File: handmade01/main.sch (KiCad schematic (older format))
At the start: 69 parts, among them CON1 MicroSD, CON2 MicroSD, J1 JACK_TRS_6PINS, P1 VOLUMN, P4 USB_OTG, P6 UART_DEBUG, Q1 1AM, SW1 POWER, SW10 R, SW11 A, SW12 B, SW13 X, SW14 Y, SW2 Reset, SW3 UP, SW4 Down, SW5 Left, SW6 Right, SW7 Select, SW8 Start, SW9 L, U1 PCM5102A, U2 PAM8403, U3 IPS_2.4_240x320_ST7789V, U4 CM3354, U5 TPS71718

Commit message: 20171130
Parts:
- J1: footprint Connectors:PJ311_3.5mm_Jack -> mylib:pj311_3.5mm
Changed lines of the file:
@@
 F 0 "J1" H 1800 10200 50  0000 C CNN
 F 1 "JACK_TRS_6PINS" H 1750 9500 50  0000 C CNN
-F 2 "Connectors:PJ311_3.5mm_Jack" H 1900 9650 50  0000 C CNN
+F 2 "mylib:pj311_3.5mm" H 1900 9650 50  0000 C CNN
 F 3 "" H 1900 9650 50  0000 C CNN
 	1    1800 9800

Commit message: 20171201
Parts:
- BAT1, P6: footprint Connectors_Molex:Molex_SPOX-5267_22-03-5035_03x2.54mm_Straight -> Connectors:GS3
- LS1, LS2: footprint Resistors_SMD:R_2010_HandSoldering -> Connectors:GS2
- U3: footprint mylib:fpc-45pin-0.5mm -> mylib:fpc-45pin-0.5mm-down
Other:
- note added: "20171201"
- note removed: "20171130"
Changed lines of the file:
@@
 handmade01
 Text Notes 13000 11050 0    60   ~ 12
-20171130
+20171201
 $Comp
 L +5V #PWR05
@@
 F 0 "U3" H 4150 1850 60  0000 C CNN
 F 1 "IPS_2.4_240x320_ST7789V" H 4700 1750 60  0000 C CNN
-F 2 "mylib:fpc-45pin-0.5mm" H 5150 1500 60  0000 C CNN
+F 2 "mylib:fpc-45pin-0.5mm-down" H 5150 1500 60  0000 C CNN
 F 3 "" H 5150 1500 60  0000 C CNN
 	1    5900 1500
@@
 F 0 "P6" H 11200 1750 50  0000 C CNN
 F 1 "UART_DEBUG" V 11300 1550 50  0000 C CNN
-F 2 "Connectors_Molex:Molex_SPOX-5267_22-03-5035_03x2.54mm_Straight" H 11200 1550 50  0000 C CNN
+F 2 "Connectors:GS3" H 11200 1550 50  0000 C CNN
 F 3 "" H 11200 1550 50  0000 C CNN
 	1    11200 1550
@@
 F 0 "LS2" H 4050 10325 50  0000 R CNN
 F 1 "SPEAKER_L" H 4050 10250 50  0000 R CNN
-F 2 "Resistors_SMD:R_2010_HandSoldering" H 4000 9900 50  0000 C CNN
+F 2 "Connectors:GS2" H 4000 9900 50  0000 C CNN
 F 3 "" H 3990 10050 50  0000 C CNN
 	1    4000 10100
@@
 F 0 "LS1" H 4050 9675 50  0000 R CNN
 F 1 "SPEAKER_R" H 4050 9600 50  0000 R CNN
-F 2 "Resistors_SMD:R_2010_HandSoldering" H 4000 9250 50  0000 C CNN
+F 2 "Connectors:GS2" H 4000 9250 50  0000 C CNN
 F 3 "" H 3990 9400 50  0000 C CNN
 	1    4000 9450
@@
 F 0 "BAT1" H 7600 10150 50  0000 L CNN
 F 1 "BAT" H 7600 10050 50  0000 L CNN
-F 2 "Connectors_Molex:Molex_SPOX-5267_22-03-5035_03x2.54mm_Straight" V 7500 10110 50  0000 C CNN
+F 2 "Connectors:GS3" V 7500 10110 50  0000 C CNN
 F 3 "" V 7500 10110 50  0000 C CNN
 	1    7500 10050

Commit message: 20171204
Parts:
- P4: footprint Connectors:USB_Micro-B -> Connectors:USB_Mini-B
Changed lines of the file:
@@
 F 0 "P4" H 6725 9675 50  0000 C CNN
 F 1 "USB_OTG" H 6400 10000 50  0000 C CNN
-F 2 "Connectors:USB_Micro-B" V 6350 9700 50  0000 C CNN
+F 2 "Connectors:USB_Mini-B" V 6350 9700 50  0000 C CNN
 F 3 "" V 6350 9700 50  0000 C CNN
 	1    6400 9800

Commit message: 20171207
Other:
- note added: "Handmade01"
- note removed: "1.0"
- note removed: "20171201"
- note removed: "handmade01"
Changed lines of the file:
@@
 EESchema Schematic File Version 2
-LIBS:main-rescue
 LIBS:power
 LIBS:device
@@
 LIBS:memory
 LIBS:xilinx
+LIBS:special
 LIBS:microcontrollers
 LIBS:dsp
@@
 LIBS:contrib
 LIBS:valves
-LIBS:switches
-LIBS:mysch
 LIBS:main-cache
-EELAYER 25 0
+EELAYER 27 0
 EELAYER END
 $Descr A3 16535 11693
@@
 Sheet 1 1
 Title ""
-Date ""
+Date "7 dec 2017"
 Rev ""
 Comp ""
@@
 Comment4 ""
 $EndDescr
-Text Notes 15420 11060 0    60   ~ 12
-1.0
 $Comp
 L CM3354 U4
@@
 	-1   0    0    1
 $EndComp
-Text Notes 12250 10950 0    98   ~ 20
-handmade01
-Text Notes 13000 11050 0    60   ~ 12
-20171201
 $Comp
 L +5V #PWR05
@@
 	0    1    1    0
 $EndComp
+Text Notes 12175 10975 0    60   ~ 12
+Handmade01
 $EndSCHEMATC

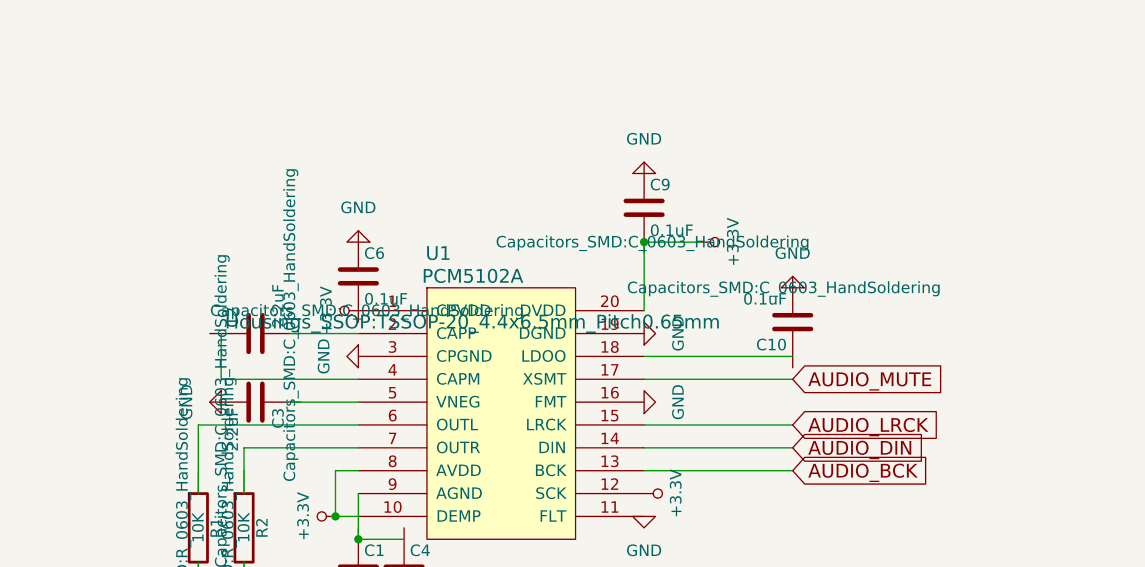
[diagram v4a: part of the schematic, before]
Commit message: 20171207
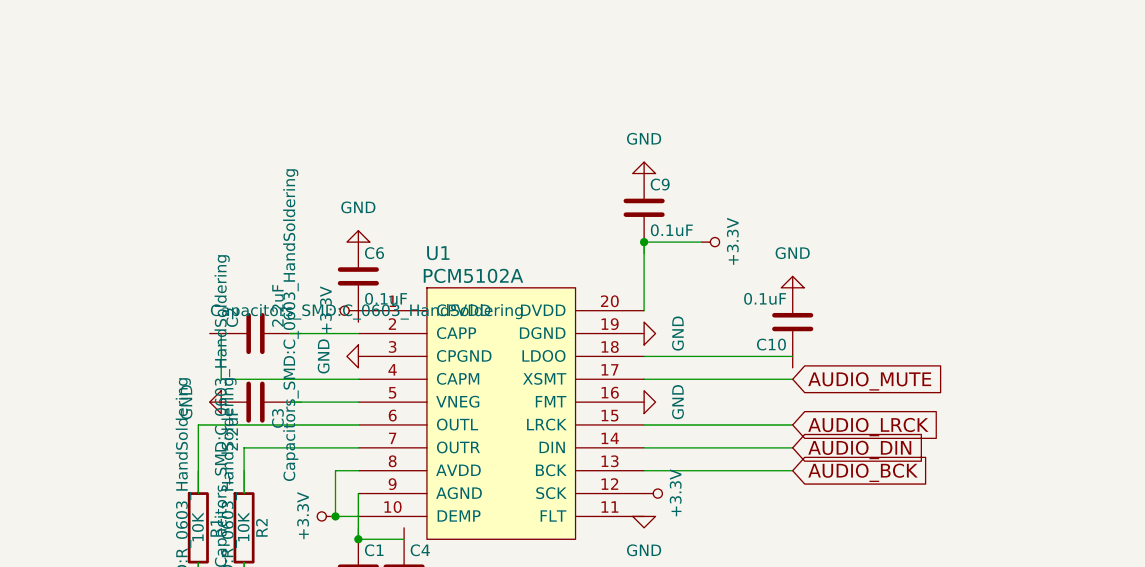
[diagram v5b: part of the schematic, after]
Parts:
- C10, C9: footprint Capacitors_SMD:C_0603_HandSoldering -> (none)
- U1: footprint Housings_SSOP:TSSOP-20_4.4x6.5mm_Pitch0.65mm -> (none)
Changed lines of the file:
@@
 F 0 "U1" H 2050 5100 60  0000 C CNN
 F 1 "PCM5102A" H 2200 5000 60  0000 C CNN
-F 2 "Housings_SSOP:TSSOP-20_4.4x6.5mm_Pitch0.65mm" H 2200 4800 60  0000 C CNN
+F 2 "" H 2200 4800 60  0000 C CNN
 F 3 "" H 2200 4800 60  0000 C CNN
 	1    2300 4450
@@
 F 0 "C10" H 3625 4200 50  0000 L CNN
 F 1 "0.1uF" H 3625 4000 50  0000 L CNN
-F 2 "Capacitors_SMD:C_0603_HandSoldering" H 3638 3950 50  0000 C CNN
+F 2 "" H 3638 3950 50  0000 C CNN
 F 3 "" H 3600 4100 50  0000 C CNN
 	1    3600 4100
@@
 F 0 "C9" H 2975 3700 50  0000 L CNN
 F 1 "0.1uF" H 2975 3500 50  0000 L CNN
-F 2 "Capacitors_SMD:C_0603_HandSoldering" H 2988 3450 50  0000 C CNN
+F 2 "" H 2988 3450 50  0000 C CNN
 F 3 "" H 2950 3600 50  0000 C CNN
 	1    2950 3600

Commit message: 20171207
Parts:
- BAT1, P6: footprint Connectors:GS3 -> (none)
- C1, C11, C12, C2, C3, C4, C5, C6, C7, C8: footprint Capacitors_SMD:C_0603_HandSoldering -> (none)
- CON1, CON2: footprint mylib:microsd -> (none)
- J1: footprint mylib:pj311_3.5mm -> (none)
- LS1, LS2: footprint Connectors:GS2 -> (none)
- P1: footprint mylib:volumn -> (none)
- P4: footprint Connectors:USB_Mini-B -> (none)
- Q1: footprint TO_SOT_Packages_SMD:SOT-23-5_HandSoldering -> (none)
- R1, R10, R11, R12, R13, R14, R15, R16, R17, R18, R19, R2, R20, R21, R22, R23, R24, R25, R26, R27, R28, R3, R4, R5, R6, R7, R8, R9: footprint Resistors_SMD:R_0603_HandSoldering -> (none)
- SW1, SW10, SW2, SW9: footprint Buttons_Switches_THT:SW_PUSH_6mm -> (none)
- SW11, SW13, SW5, SW6: footprint mylib:dpad-h -> (none)
- SW12, SW14, SW3, SW4: footprint mylib:dpad-v -> (none)
- SW7, SW8: footprint Buttons_Switches_SMD:SW_SPST_TL3342 -> (none)
- U2: footprint Housings_SSOP:SOP-16_4.4x10.4mm_Pitch1.27mm -> (none)
- U3: footprint mylib:fpc-45pin-0.5mm-down -> (none)
- U4: footprint mylib:cm3354 -> (none)
- U5: footprint mylib:sc-70-5 -> (none)
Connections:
- wire segments 40 -> 39
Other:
- moved on the sheet: C1, C10, C11, C12, C2, C3, C4, C5, C6, C7, C8, C9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

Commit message: 20171208
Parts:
- SW1: value POWER -> Power
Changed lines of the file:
@@
 Sheet 1 1
 Title ""
-Date "7 dec 2017"
+Date "8 dec 2017"
 Rev ""
 Comp ""
@@
 P 11800 9100
 F 0 "SW1" H 11850 9200 50  0000 L CNN
-F 1 "POWER" H 11800 9040 50  0000 C CNN
+F 1 "Power" H 11800 9040 50  0000 C CNN
 F 2 "" H 11800 9300 50  0001 C CNN
 F 3 "" H 11800 9300 50  0001 C CNN
